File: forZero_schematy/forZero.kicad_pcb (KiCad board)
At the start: 2 copper layers, 70 x 70 mm, 96 parts, among them IC1 NCV21872DMR2G, IC2 MCP4661-103E_ST, IC3 STM32F105RBT6, IC4 AP7347DQ-33W5-7, IC5 MCP2562-E_SN, J1 USB_C_Receptacle_USB2.0_16P, J2 43045-0800, J3 43045-0621, J4 43045-0400, J5 Barrel_Jack_Switch, Q1 AO3400A, Q10 AO3400A, Q2 AO3400A, Q3 AO3400A, Q4 AO3400A, Q5 AO3400A, Q6 AO3400A, Q7 AO3400A, Q8 AO3400A, Q9 AO3400A, Y1 25MHz

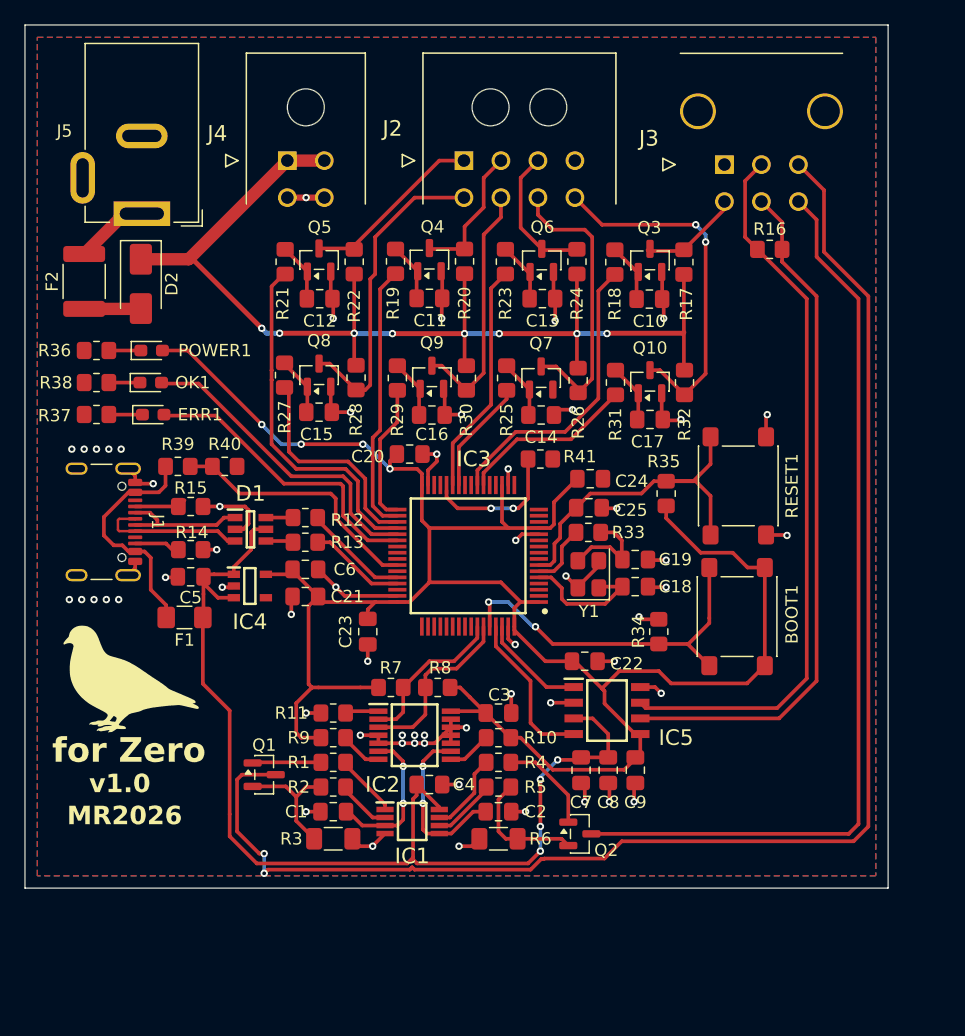
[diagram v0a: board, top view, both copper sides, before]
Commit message: Wprowadzenie poprawek PCB
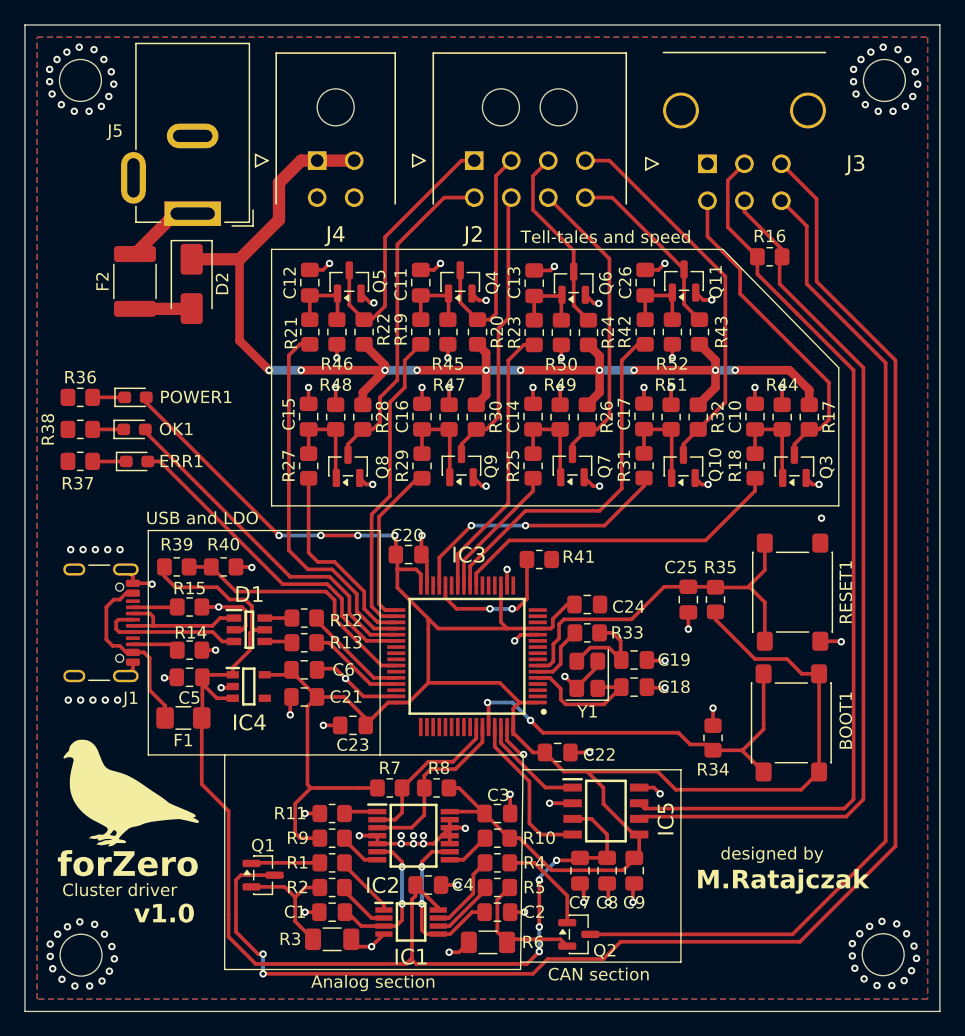
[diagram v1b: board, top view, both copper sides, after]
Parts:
- added C26: 100n, Capacitor_SMD:C_0805_2012Metric_Pad1.18x1.45mm_HandSolder, F.Cu at (119.3, 75.9)
- added Q11: AO3400A, Package_TO_SOT_SMD:SOT-23, F.Cu at (122.5, 75.8)
- added R42: 100R, Resistor_SMD:R_0805_2012Metric_Pad1.20x1.40mm_HandSolder, F.Cu at (119.3, 79.9)
- added R43: 9.1k, Resistor_SMD:R_0805_2012Metric_Pad1.20x1.40mm_HandSolder, F.Cu at (123.7, 79.9)
- added R44: 9.1k, Resistor_SMD:R_0805_2012Metric_Pad1.20x1.40mm_HandSolder, F.Cu at (130.4, 86.8)
- added R45: 9.1k, Resistor_SMD:R_0805_2012Metric_Pad1.20x1.40mm_HandSolder, F.Cu at (103.3, 79.9)
- added R46: 9.1k, Resistor_SMD:R_0805_2012Metric_Pad1.20x1.40mm_HandSolder, F.Cu at (94.3, 79.9)
- added R47: 9.1k, Resistor_SMD:R_0805_2012Metric_Pad1.20x1.40mm_HandSolder, F.Cu at (103.4, 86.8)
- added R48: 9.1k, Resistor_SMD:R_0805_2012Metric_Pad1.20x1.40mm_HandSolder, F.Cu at (94.2, 86.8)
- added R49: 9.1k, Resistor_SMD:R_0805_2012Metric_Pad1.20x1.40mm_HandSolder, F.Cu at (112.4, 86.8)
- added R50: 9.1k, Resistor_SMD:R_0805_2012Metric_Pad1.20x1.40mm_HandSolder, F.Cu at (112.5, 79.9)
- added R51: 9.1k, Resistor_SMD:R_0805_2012Metric_Pad1.20x1.40mm_HandSolder, F.Cu at (121.4, 86.8)
- added R52: 9.1k, Resistor_SMD:R_0805_2012Metric_Pad1.20x1.40mm_HandSolder, F.Cu at (121.5, 79.9)
- R18, R19, R21, R23, R25, R27, R29, R31: value 1k -> 100R
- moved Q3 20.4 mm to (131.4, 90.8)
- moved R18 20.1 mm to (128.2, 90.8)
- moved R17 16.2 mm to (132.6, 86.8), turned to -90 degrees
- moved C10 12.8 mm to (128.2, 86.8), turned to -90 degrees
- moved C25 11.0 mm to (122.8, 101.6), turned to -90 degrees
- moved C24 10.2 mm to (114.6, 102.0)
- moved RESET1 9.68 mm to (131.2, 101.0)
- moved BOOT1 9.68 mm to (131.2, 111.6)
- moved R34 9.68 mm to (124.8, 112.8)
- moved R35 9.48 mm to (125.0, 101.6)
- moved R6 8.44 mm to (106.5, 129.4)
- moved J1 8.18 mm to (74.1, 103.5)
- moved C1 8.15 mm to (93.9, 127.0)
- moved C18 8.15 mm to (118.4, 108.7)
- moved C19 8.15 mm to (118.4, 106.5)
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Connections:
- net CLUSTER_BREAK_PADS renamed CLUSTER_BRAKE_PADS
- C10 pad 1: Net-(Q3-G) -> GND
- C10 pad 2: GND -> Net-(Q3-G)
- C12 pad 1: Net-(Q5-G) -> GND
- C12 pad 2: GND -> Net-(Q5-G)
- C13 pad 1: Net-(Q6-G) -> GND
- C13 pad 2: GND -> Net-(Q6-G)
- C14 pad 1: Net-(Q7-G) -> GND
- C14 pad 2: GND -> Net-(Q7-G)
- C15 pad 1: Net-(Q8-G) -> GND
- C15 pad 2: GND -> Net-(Q8-G)
- C16 pad 1: Net-(Q9-G) -> GND
- C16 pad 2: GND -> Net-(Q9-G)
- C17 pad 1: Net-(Q10-G) -> GND
- C17 pad 2: GND -> Net-(Q10-G)
- F1 pad 2: 5V_USB -> Net-(F1-Pad2)
- IC3 pad 22: SENSOR -> unconnected-(IC3-PA6-Pad22)
- IC3 pad 24: unconnected-(IC3-PC4-Pad24) -> TCR
- IC3 pad 25: unconnected-(IC3-PC5-Pad25) -> BRAKE_PADS
- IC3 pad 26: BREAK_PADS -> ABS
- IC3 pad 27: ABS -> unconnected-(IC3-PB1-Pad27)
- IC3 pad 29: unconnected-(IC3-PB10-Pad29) -> SENSOR
- J1 pad A4: 5V_USB -> Net-(F1-Pad2)
- J1 pad A9: 5V_USB -> Net-(F1-Pad2)
- J1 pad B4: 5V_USB -> Net-(F1-Pad2)
- J1 pad B9: 5V_USB -> Net-(F1-Pad2)
- J2 pad 4: unconnected-(J2-Pad4) -> CLUSTER_SENSOR
- J2 pad 8: CLUSTER_SENSOR -> CLUSTER_TCR
- R25 pad 1: BREAK_PADS -> BRAKE_PADS
- R39 pad 1: 5V_USB -> 5V
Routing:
- net TCR: track 0.00 -> 29.3 mm
- net 5V_USB: track 19.0 -> 0.00 mm
- net CLUSTER_SPEED: track 8.06 -> 26.5 mm
- net CLUSTER_CAN_L: track 56.3 -> 71.6 mm
- net CLUSTER_CAN_H: track 59.0 -> 74.2 mm
- net CLUSTER_TCR: track 0.00 -> 15.0 mm
- net Net-(F1-Pad2): track 0.00 -> 14.8 mm
- net 5V: track 86.9 -> 98.6 mm
- net BRAKE_PADS: track 0.00 -> 11.0 mm
- net 3V3: track 173.6 -> 184.2 mm
- net BREAK_PADS: track 9.29 -> 0.00 mm
- net GND: track 111.2 -> 119.4 mm, vias 59 -> 138
- net CLUSTER_AIR_BAG: track 11.3 -> 19.3 mm
- net CLUSTER_TEMP_LVL: track 74.5 -> 82.5 mm
- net CLUSTER_FUEL_LVL: track 118.8 -> 126.8 mm
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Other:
- board size 70 x 70 mm -> 74.2 x 80 mm
- board text added: "1- TCR 2- SENSOR 3- BRAKE PADS 4- ABS 5- COOL LVL 6- AIR BAG 7- WIPER FLUID 8- BRAKES"
- board text added: "Analog section"
- board text added: "CAN section"
- board text added: "Cluster driver"
- board text added: "M.Ratajczak"
- board text added: "Tell-tales and speed"
- board text added: "USB and LDO"
- board text added: "designed by"
- board text added: "forZero"
- board text removed: "1- SENSOR 2- N/A 3- BREAK PADS 4- ABS 5- COOL LVL 6- AIR BAG 7- WIPER FLUID 8- BREAKS"
- board text removed: "MR2026"
- board text removed: "for Zero"
